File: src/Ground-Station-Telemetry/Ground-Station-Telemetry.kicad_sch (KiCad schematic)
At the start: 36 parts, among them J1 Jumper_NO, P1 3220-20-0200-00, U1 STM32H750VBTx, U2 LMS8117AMP-3.3_NOPB, Y1 ECS-240-18-33-JGN-TR

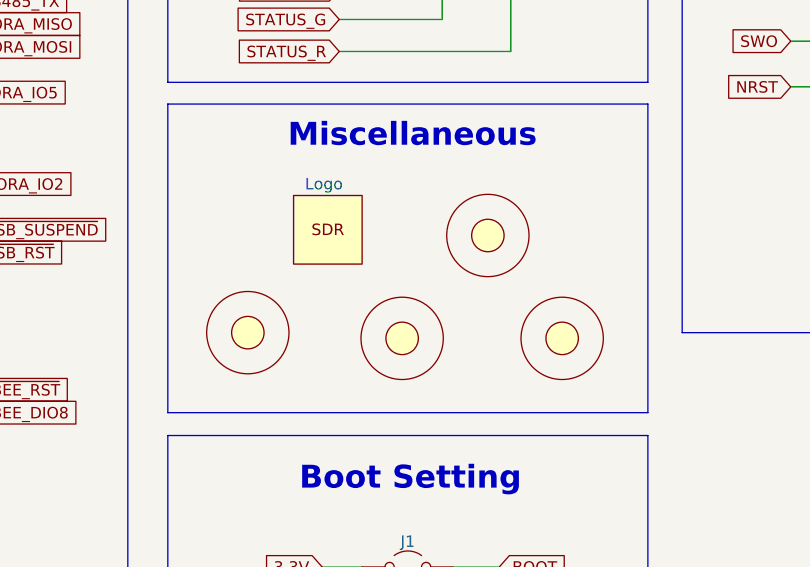
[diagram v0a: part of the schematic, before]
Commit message: finished initial rev 2 routing
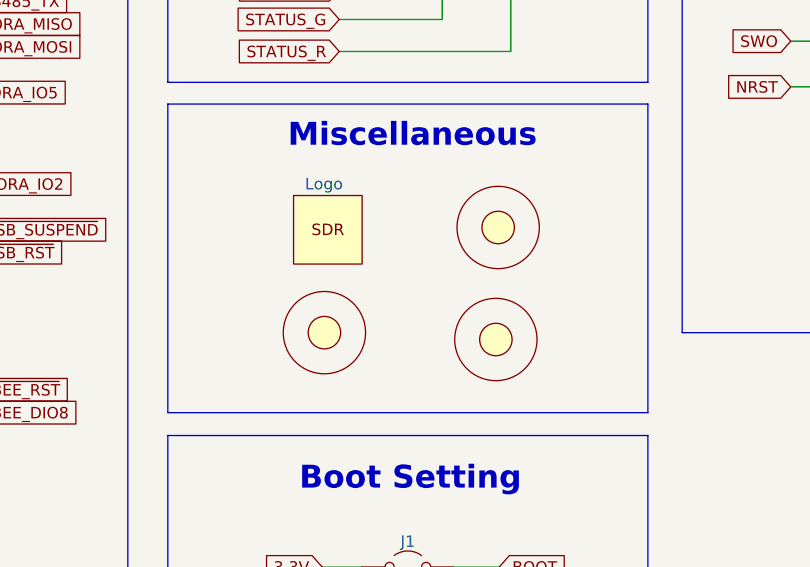
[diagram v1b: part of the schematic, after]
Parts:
- removed H3: Mounting-Hole, Engine-Controller:MountingHole_4.3mm_M4_DIN965, symbol Ground-Station-Telemetry:Mounting-Hole
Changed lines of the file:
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@@
-    )
-  )
-  (symbol (lib_id "Ground-Station-Telemetry:Mounting-Hole") (at 156.845 150.495 0) (unit 1)
-    (in_bom yes) (on_board yes) (dnp no) (fields_autoplaced)
-    (property "Reference" "H3" (at 156.845 144.145 0)
-      (effects (font (size 1.27 1.27)) hide)
-    )
-    (property "Value" "Mounting-Hole" (at 156.845 155.575 0)
-      (effects (font (size 1.27 1.27)) hide)
-    )
-    (property "Footprint" "Engine-Controller:MountingHole_4.3mm_M4_DIN965" (at 156.845 150.495 0)
-      (effects (font (size 1.27 1.27)) hide)
-    )
-    (property "Datasheet" "" (at 156.845 150.495 0)
-      (effects (font (size 1.27 1.27)) hide)
-    )
-    (instances
-      (project "Ground-Station-Telemetry"
-        (path "/8e3fff47-8adf-433e-a9ef-a2ec6a2108a7"
-          (reference "H3") (unit 1)
-        )
-      )
     )
   )
@@
     )
   )
-  (symbol (lib_id "Ground-Station-Telemetry:Mounting-Hole") (at 165.1 161.925 0) (unit 1)
-    (in_bom yes) (on_board yes) (dnp no) (fields_autoplaced)
-    (property "Reference" "H4" (at 165.1 155.575 0)
-      (effects (font (size 1.27 1.27)) hide)
-    )
-    (property "Value" "Mounting-Hole" (at 165.1 167.005 0)
-      (effects (font (size 1.27 1.27)) hide)
-    )
-    (property "Footprint" "Engine-Controller:MountingHole_4.3mm_M4_DIN965" (at 165.1 161.925 0)
-      (effects (font (size 1.27 1.27)) hide)
-    )
-    (property "Datasheet" "" (at 165.1 161.925 0)
+  (symbol (lib_id "Ground-Station-Telemetry:Mounting-Hole") (at 157.988 149.606 0) (unit 1)
+    (in_bom yes) (on_board yes) (dnp no) (fields_autoplaced)
+    (property "Reference" "H4" (at 157.988 143.256 0)
+      (effects (font (size 1.27 1.27)) hide)
+    )
+    (property "Value" "Mounting-Hole" (at 157.988 154.686 0)
+      (effects (font (size 1.27 1.27)) hide)
+    )
+    (property "Footprint" "Engine-Controller:MountingHole_4.3mm_M4_DIN965" (at 157.988 149.606 0)
+      (effects (font (size 1.27 1.27)) hide)
+    )
+    (property "Datasheet" "" (at 157.988 149.606 0)
       (effects (font (size 1.27 1.27)) hide)
     )
@@
     )
   )
-  (symbol (lib_id "Ground-Station-Telemetry:Mounting-Hole") (at 130.175 161.29 0) (unit 1)
-    (in_bom yes) (on_board yes) (dnp no) (fields_autoplaced)
-    (property "Reference" "H1" (at 130.175 154.94 0)
-      (effects (font (size 1.27 1.27)) hide)
-    )
-    (property "Value" "Mounting-Hole" (at 130.175 166.37 0)
-      (effects (font (size 1.27 1.27)) hide)
-    )
-    (property "Footprint" "Engine-Controller:MountingHole_4.3mm_M4_DIN965" (at 130.175 161.29 0)
-      (effects (font (size 1.27 1.27)) hide)
-    )
-    (property "Datasheet" "" (at 130.175 161.29 0)
+  (symbol (lib_id "Ground-Station-Telemetry:Mounting-Hole") (at 138.684 161.29 0) (unit 1)
+    (in_bom yes) (on_board yes) (dnp no) (fields_autoplaced)
+    (property "Reference" "H1" (at 138.684 154.94 0)
+      (effects (font (size 1.27 1.27)) hide)
+    )
+    (property "Value" "Mounting-Hole" (at 138.684 166.37 0)
+      (effects (font (size 1.27 1.27)) hide)
+    )
+    (property "Footprint" "Engine-Controller:MountingHole_4.3mm_M4_DIN965" (at 138.684 161.29 0)
+      (effects (font (size 1.27 1.27)) hide)
+    )
+    (property "Datasheet" "" (at 138.684 161.29 0)
       (effects (font (size 1.27 1.27)) hide)
     )
@@
     )
   )
-  (symbol (lib_id "Ground-Station-Telemetry:Mounting-Hole") (at 147.32 161.925 0) (unit 1)
-    (in_bom yes) (on_board yes) (dnp no) (fields_autoplaced)
-    (property "Reference" "H2" (at 147.32 155.575 0)
-      (effects (font (size 1.27 1.27)) hide)
-    )
-    (property "Value" "Mounting-Hole" (at 147.32 167.005 0)
-      (effects (font (size 1.27 1.27)) hide)
-    )
-    (property "Footprint" "Engine-Controller:MountingHole_4.3mm_M4_DIN965" (at 147.32 161.925 0)
-      (effects (font (size 1.27 1.27)) hide)
-    )
-    (property "Datasheet" "" (at 147.32 161.925 0)
-      (effects (font (size 1.27 1.27)) hide)
-    )
+  (symbol (lib_id "Ground-Station-Telemetry:Mounting-Hole") (at 157.734 162.052 0) (unit 1)
+    (in_bom yes) (on_board yes) (dnp no) (fields_autoplaced)
+    (property "Reference" "H2" (at 157.734 155.702 0)
+      (effects (font (size 1.27 1.27)) hide)
+    )
+    (property "Value" "Mounting-Hole" (at 157.734 167.132 0)
+      (effects (font (size 1.27 1.27)) hide)
+    )
+    (property "Footprint" "Engine-Controller:MountingHole_4.3mm_M4_DIN965" (at 157.734 162.052 0)
+      (effects (font (size 1.27 1.27)) hide)
+    )
+    (property "Datasheet" "" (at 157.734 162.052 0)
+      (effects (font (size 1.27 1.27)) hide)
+    )
